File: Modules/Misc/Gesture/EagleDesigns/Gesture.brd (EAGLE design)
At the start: 100 x 80 mm, 13 parts, among them U2 ATMEGA328P_TQFP, U3 LSM9DS1

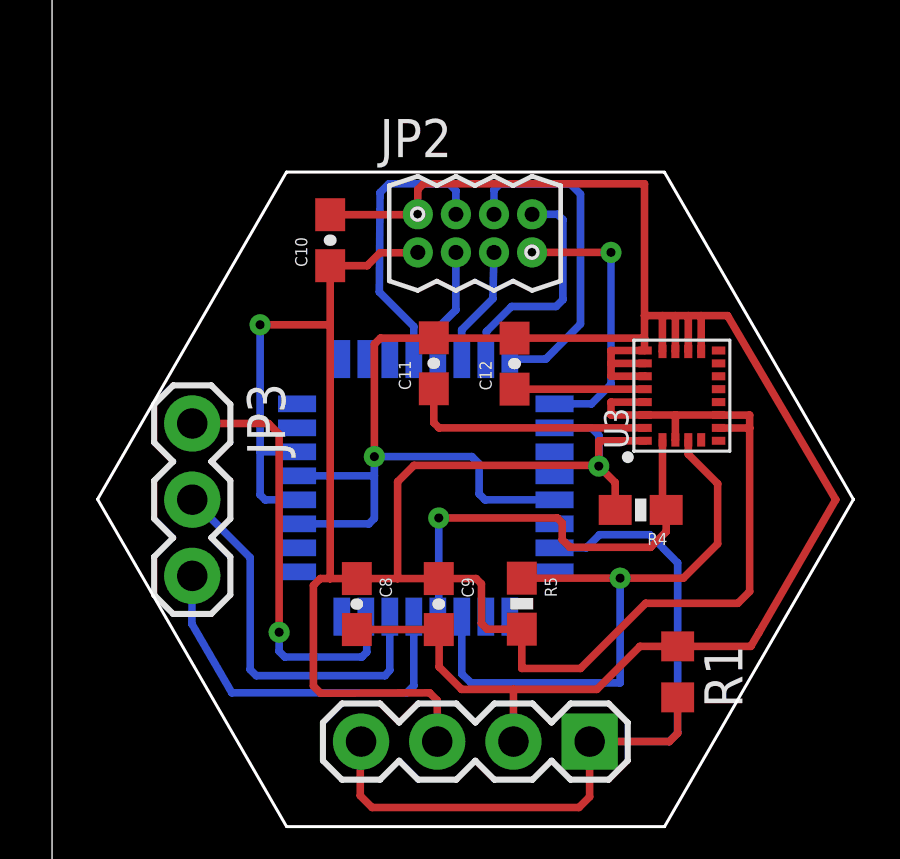
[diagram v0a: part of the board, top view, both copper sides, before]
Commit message: unknown changes! :(
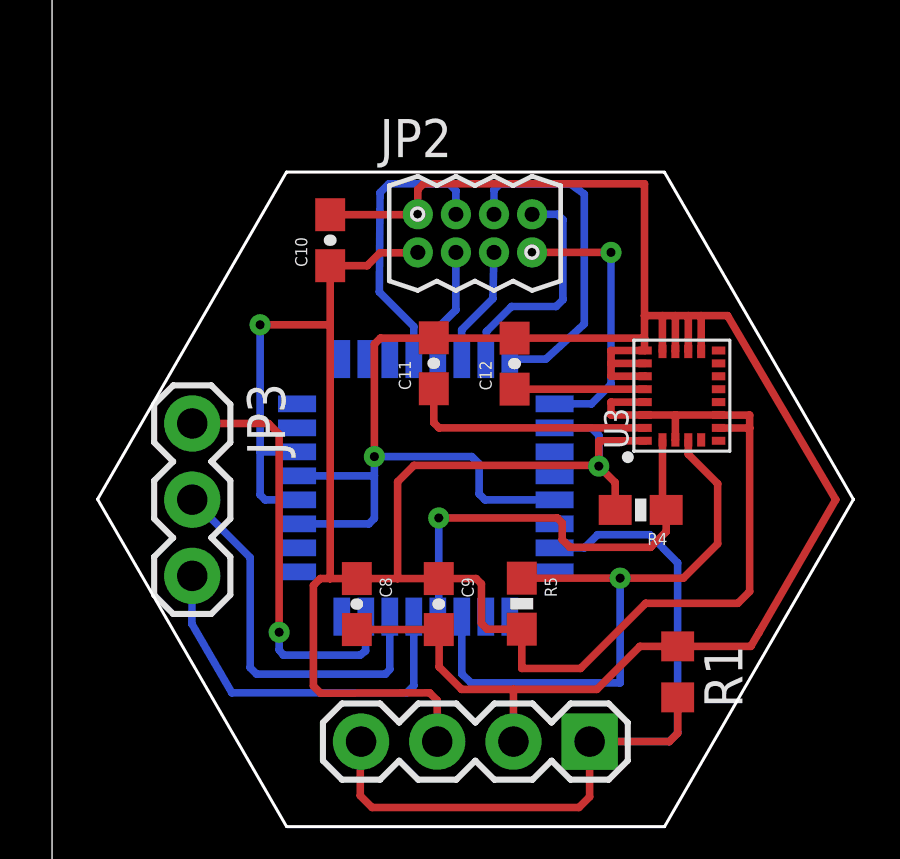
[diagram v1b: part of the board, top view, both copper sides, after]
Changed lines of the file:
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@@
 <grid distance="0.0127" unitdist="mm" unit="mm" style="lines" multiple="1" display="no" altdistance="0.00635" altunitdist="mm" altunit="mm"/>
 <layers>
-<layer number="1" name="Top" color="4" fill="1" visible="yes" active="yes"/>
+<layer number="1" name="Top" color="4" fill="1" visible="no" active="yes"/>
 <layer number="2" name="Route2" color="1" fill="3" visible="no" active="no"/>
 <layer number="15" name="Route15" color="4" fill="6" visible="no" active="no"/>
@@
 <wire x1="10.2743" y1="2.286" x2="10.2743" y2="4.064" width="0.254" layer="1"/>
 <wire x1="10.2743" y1="4.064" x2="10.2997" y2="4.0894" width="0.254" layer="1"/>
-<wire x1="16.7513" y1="10.5476" x2="17.812" y2="10.5476" width="0.254" layer="16"/>
-<wire x1="17.812" y1="10.5476" x2="18.2499" y2="10.9855" width="0.254" layer="16"/>
-<wire x1="18.2499" y1="10.9855" x2="19.9263" y2="10.9855" width="0.254" layer="16"/>
+<wire x1="16.7513" y1="10.5476" x2="17.7485" y2="10.5476" width="0.254" layer="16"/>
+<wire x1="17.7485" y1="10.5476" x2="18.1864" y2="10.9855" width="0.254" layer="16"/>
+<wire x1="18.1864" y1="10.9855" x2="19.9263" y2="10.9855" width="0.254" layer="16"/>
 <wire x1="19.9263" y1="10.9855" x2="20.8534" y2="10.0457" width="0.254" layer="16"/>
 <wire x1="20.8534" y1="10.0457" x2="20.8534" y2="4.3688" width="0.254" layer="16"/>
@@
 <wire x1="14.732" y1="22.479" x2="14.9352" y2="22.6822" width="0.254" layer="16"/>
 <wire x1="14.9352" y1="22.6822" x2="17.272" y2="22.6822" width="0.254" layer="16"/>
-<wire x1="17.272" y1="22.6822" x2="17.6149" y2="22.3393" width="0.254" layer="16"/>
-<wire x1="17.6149" y1="22.3393" x2="17.6149" y2="18.0086" width="0.254" layer="16"/>
-<wire x1="17.6149" y1="18.0086" x2="16.4592" y2="16.8402" width="0.254" layer="16"/>
+<wire x1="17.272" y1="22.6822" x2="17.7419" y2="22.3393" width="0.254" layer="16"/>
+<wire x1="17.7419" y1="22.3393" x2="17.7419" y2="18.0086" width="0.254" layer="16"/>
+<wire x1="17.7419" y1="18.0086" x2="16.4592" y2="16.8402" width="0.254" layer="16"/>
 <wire x1="16.4592" y1="16.8402" x2="15.2587" y2="16.8402" width="0.254" layer="16"/>
 </signal>
@@
 <contactref element="U2" pad="30"/>
 <contactref element="JP3" pad="2"/>
-<wire x1="11.2587" y1="8.255" x2="11.2587" y2="6.4708" width="0.254" layer="16"/>
-<wire x1="11.2587" y1="6.4708" x2="11.0998" y2="6.2865" width="0.254" layer="16"/>
-<wire x1="11.0998" y1="6.2865" x2="6.8072" y2="6.2865" width="0.254" layer="16"/>
-<wire x1="6.8072" y1="6.2865" x2="6.604" y2="6.4897" width="0.254" layer="16"/>
-<wire x1="6.604" y1="6.4897" x2="6.604" y2="10.2235" width="0.254" layer="16"/>
+<wire x1="11.2587" y1="8.255" x2="11.2587" y2="6.4962" width="0.254" layer="16"/>
+<wire x1="11.2587" y1="6.4962" x2="11.1125" y2="6.3373" width="0.254" layer="16"/>
+<wire x1="11.1125" y1="6.3373" x2="6.8199" y2="6.3373" width="0.254" layer="16"/>
+<wire x1="6.8199" y1="6.3373" x2="6.604" y2="6.5532" width="0.254" layer="16"/>
+<wire x1="6.604" y1="6.5532" x2="6.604" y2="10.2235" width="0.254" layer="16"/>
 <wire x1="6.604" y1="10.2235" x2="4.6736" y2="12.1539" width="0.254" layer="16"/>
 </signal>
@@
 <wire x1="7.5692" y1="14.3383" x2="7.5692" y2="7.7343" width="0.254" layer="1"/>
 <via x="7.5692" y="7.7343" extent="1-16" drill="0.3"/>
-<wire x1="7.5692" y1="7.7343" x2="7.5692" y2="7.0993" width="0.254" layer="16"/>
-<wire x1="7.5692" y1="7.0993" x2="7.7597" y2="6.9088" width="0.254" layer="16"/>
-<wire x1="7.7597" y1="6.9088" x2="10.3251" y2="6.9088" width="0.254" layer="16"/>
-<wire x1="10.3251" y1="6.9088" x2="10.4902" y2="7.0739" width="0.254" layer="16"/>
-<wire x1="10.4902" y1="7.0739" x2="10.4902" y2="7.7917" width="0.254" layer="16"/>
-<wire x1="10.4902" y1="7.7917" x2="10.4587" y2="8.255" width="0.254" layer="16"/>
+<wire x1="7.5692" y1="7.7343" x2="7.5692" y2="7.1501" width="0.254" layer="16"/>
+<wire x1="7.5692" y1="7.1501" x2="7.7089" y2="6.9723" width="0.254" layer="16"/>
+<wire x1="7.7089" y1="6.9723" x2="10.2743" y2="6.9723" width="0.254" layer="16"/>
+<wire x1="10.2743" y1="6.9723" x2="10.4521" y2="7.112" width="0.254" layer="16"/>
+<wire x1="10.4521" y1="7.112" x2="10.4521" y2="7.8298" width="0.254" layer="16"/>
+<wire x1="10.4521" y1="7.8298" x2="10.4587" y2="8.255" width="0.254" layer="16"/>
 </signal>
 </signals>
